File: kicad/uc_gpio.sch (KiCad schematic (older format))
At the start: 1 part, among them U1_501 TMS320F28388DZWTS

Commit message: begin PCB!! it's amess but IT IS
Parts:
- U1_501: footprint (none) -> servo:BGA337CP80_19X19_1600X1600X140B50N
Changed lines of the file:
@@
 F 0 "U1_501" H 5900 10873 60  0000 C CNN
 F 1 "TMS320F28388DZWTS" H 5900 10775 50  0000 C CNN
-F 2 "" H 5900 6300 50  0001 C CNN
+F 2 "servo:BGA337CP80_19X19_1600X1600X140B50N" H 5900 6300 50  0001 C CNN
 F 3 "../doc/datasheets/tms320f28388d_datasheet.pdf" H 5900 6300 50  0001 C CNN
 F 4 "TMS320F28388DZWTS" V 4300 3200 60  0001 C CNN "PartNumber"

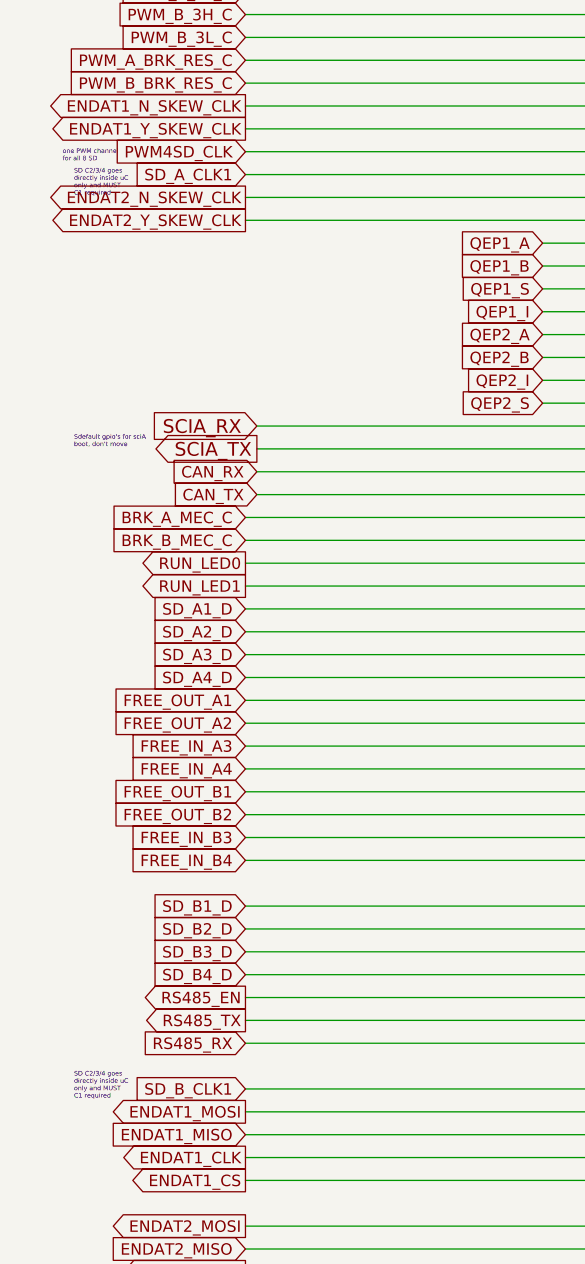
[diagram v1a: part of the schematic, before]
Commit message: I've passed all footprin to layout BUT...
I've passed all, first glance... I need to confirm in details a lot of
things. The objetive for these is to have an aproximation of the size
I'll need to make the board.. then I choose the final detailed footprint
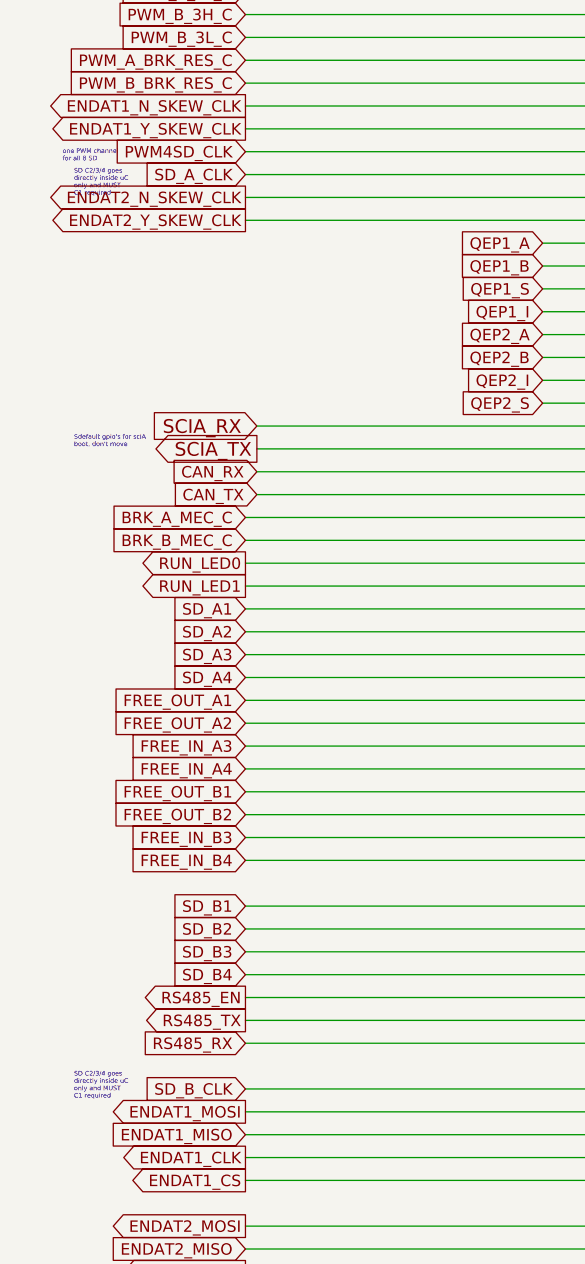
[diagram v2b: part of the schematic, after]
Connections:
- net SD_A1_D renamed SD_A1
- net SD_A2_D renamed SD_A2
- net SD_A3_D renamed SD_A3
- net SD_A4_D renamed SD_A4
- net SD_A_CLK1 renamed SD_A_CLK
- net SD_B1_D renamed SD_B1
- net SD_B2_D renamed SD_B2
- net SD_B3_D renamed SD_B3
- net SD_B4_D renamed SD_B4
- net SD_B_CLK1 renamed SD_B_CLK
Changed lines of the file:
@@
 $Descr A3 16535 11693
 encoding utf-8
-Sheet 14 18
+Sheet 14 19
 Title "gpio"
 Date "2020-01-09"
@@
 	3200 5000 4800 5000
 Text GLabel 3150 5700 0    50   Input ~ 0
-SD_A1_D
+SD_A1
 Text GLabel 3150 5800 0    50   Input ~ 0
-SD_A2_D
+SD_A2
 Text GLabel 3150 5900 0    50   Input ~ 0
-SD_A3_D
+SD_A3
 Text GLabel 3150 6000 0    50   Input ~ 0
-SD_A4_D
+SD_A4
 Text GLabel 3150 3300 0    50   Input ~ 0
 PWM_A_BRK_RES_C
@@
 PWM_B_BRK_RES_C
 Text GLabel 3150 7000 0    50   Input ~ 0
-SD_B1_D
+SD_B1
 Text GLabel 3150 7100 0    50   Input ~ 0
-SD_B2_D
+SD_B2
 Text GLabel 3150 7200 0    50   Input ~ 0
-SD_B3_D
+SD_B3
 Wire Wire Line
 	3150 7000 4800 7000
@@
 	3150 3800 4800 3800
 Text GLabel 3150 3800 0    50   Input ~ 0
-SD_A_CLK1
+SD_A_CLK
 Text GLabel 3150 3700 0    50   Input ~ 0
 PWM4SD_CLK
@@
 SD C2/3/4 goes\ndirectly inside uC\nonly and MUST  \nC1 required
 Text GLabel 3150 7800 0    50   Input ~ 0
-SD_B_CLK1
+SD_B_CLK
 Wire Wire Line
 	3150 7300 4800 7300
 Text GLabel 3150 7300 0    50   Input ~ 0
-SD_B4_D
+SD_B4
 Text GLabel 3150 7600 0    50   Input ~ 0
 RS485_RX
